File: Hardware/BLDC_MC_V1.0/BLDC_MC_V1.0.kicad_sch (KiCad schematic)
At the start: 0 parts

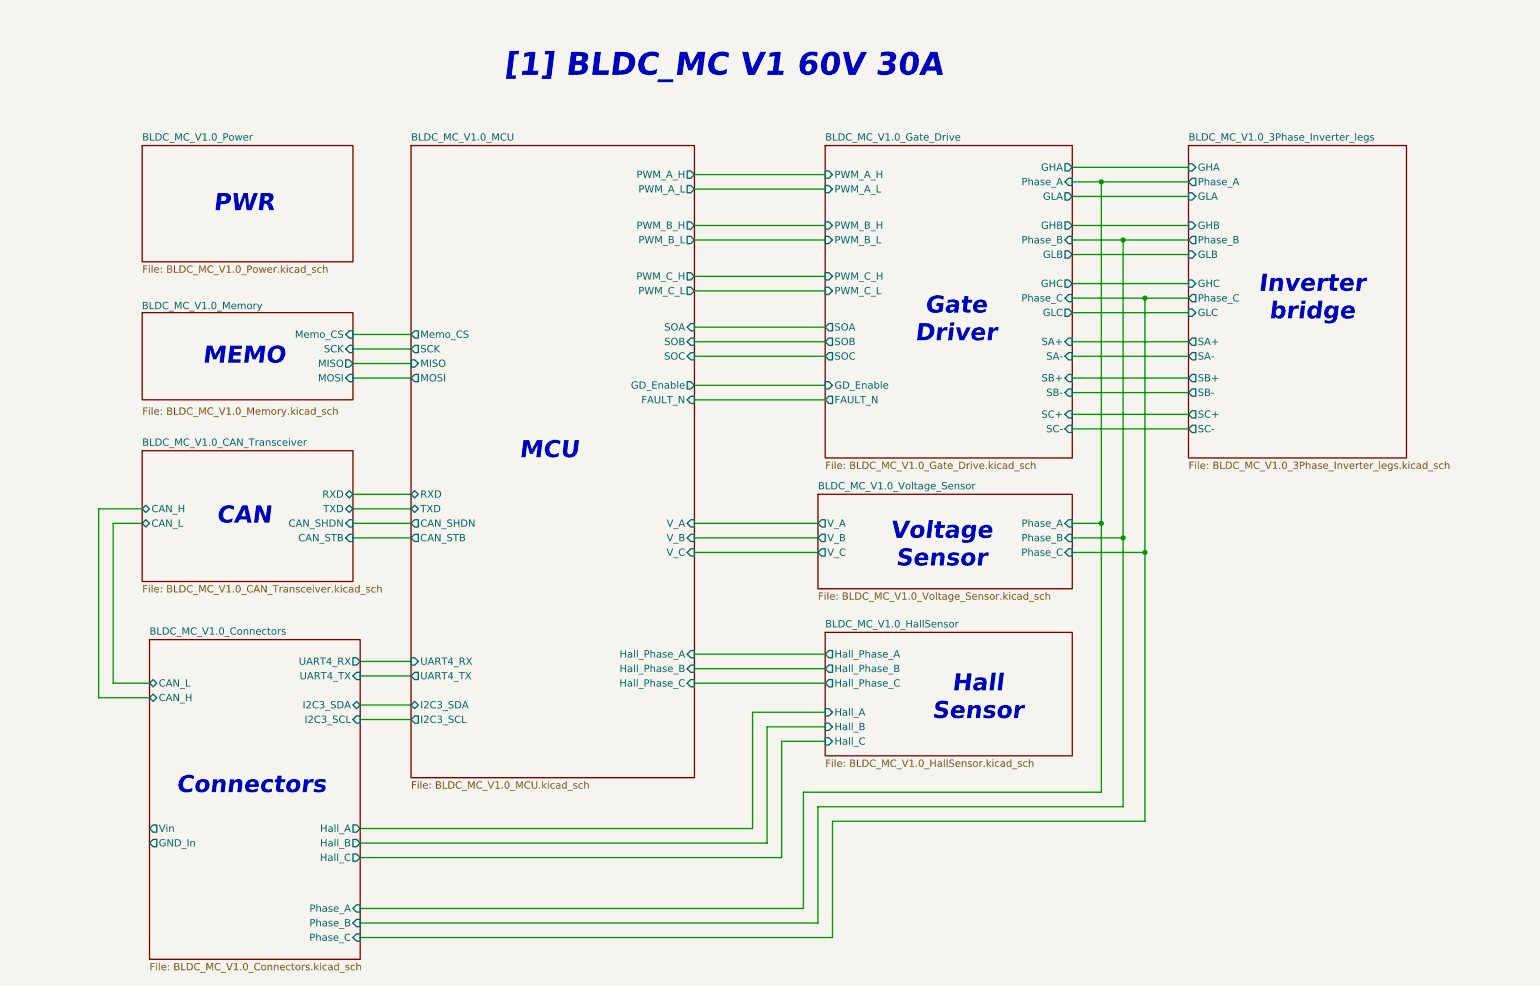
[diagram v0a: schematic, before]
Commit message: Solve all errors and wornings in project
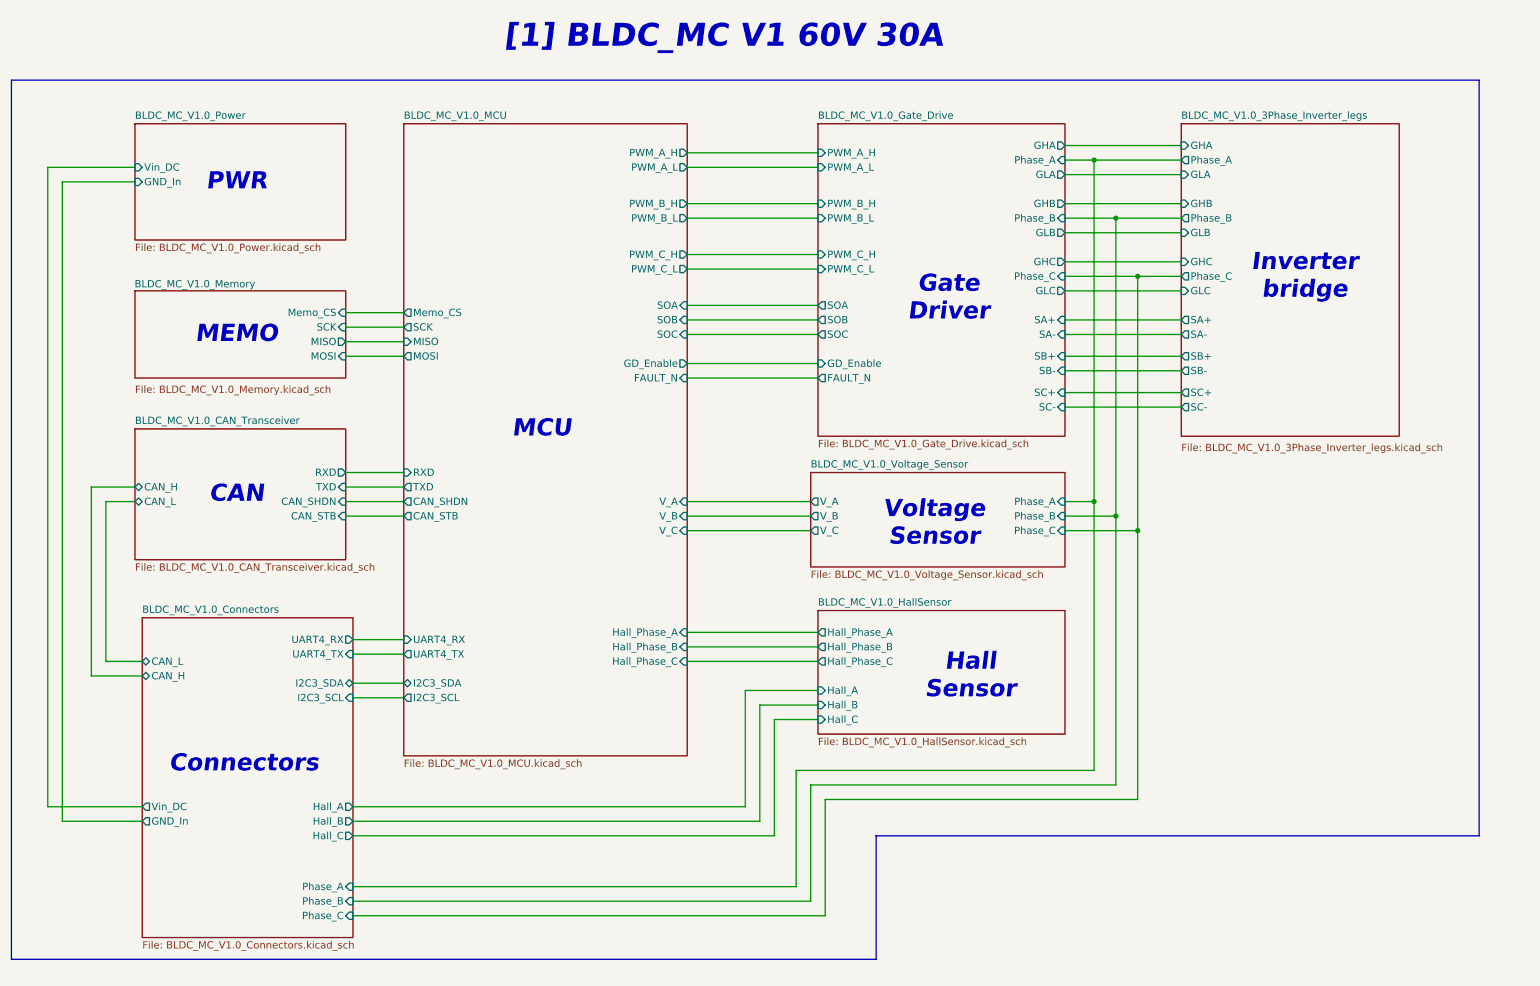
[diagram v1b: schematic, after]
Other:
- sheet BLDC_MC_V1.0_Connectors ports: added Vin_DC; removed Vin
- sheet BLDC_MC_V1.0_Power ports: added GND_In, Vin_DC; removed none
